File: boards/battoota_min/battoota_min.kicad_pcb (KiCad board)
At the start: 2 copper layers, 110.9 x 82.1 mm, 21 parts

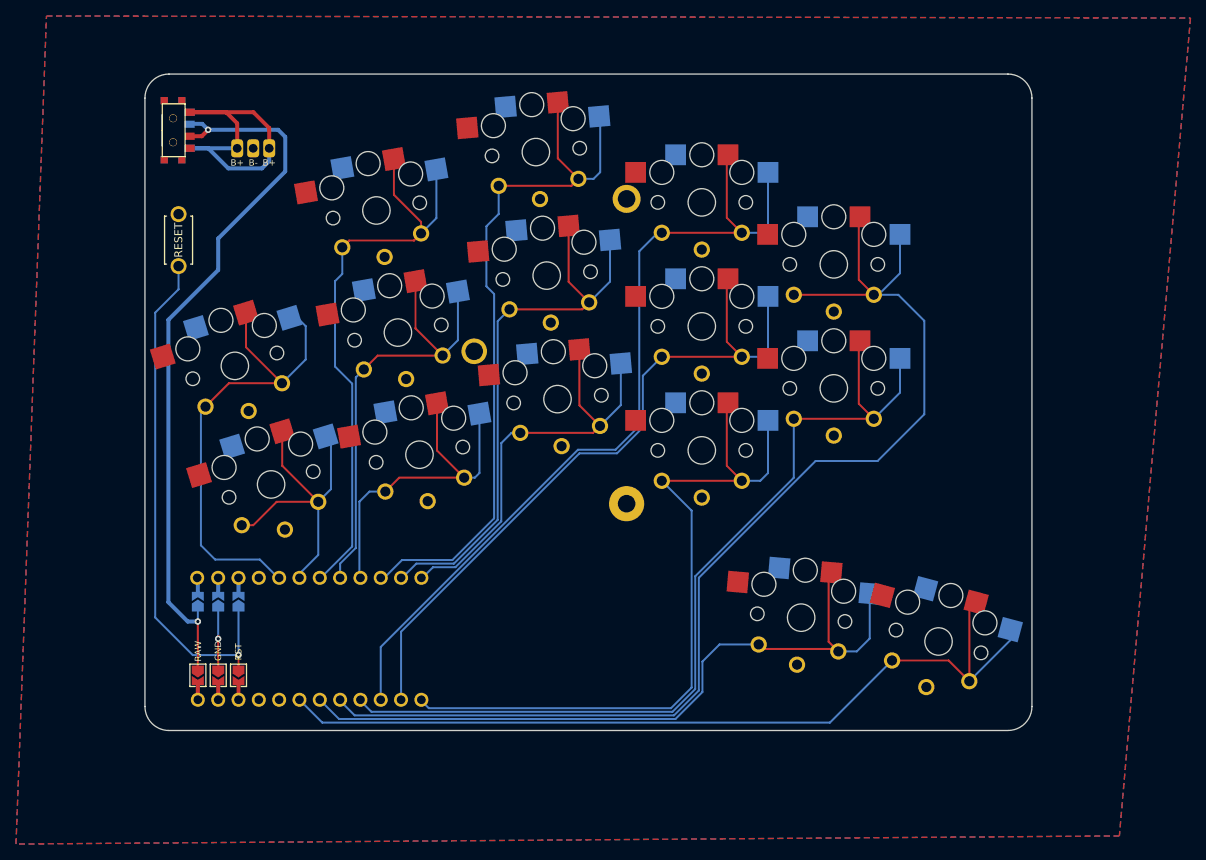
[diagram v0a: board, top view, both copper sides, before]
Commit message: min changes
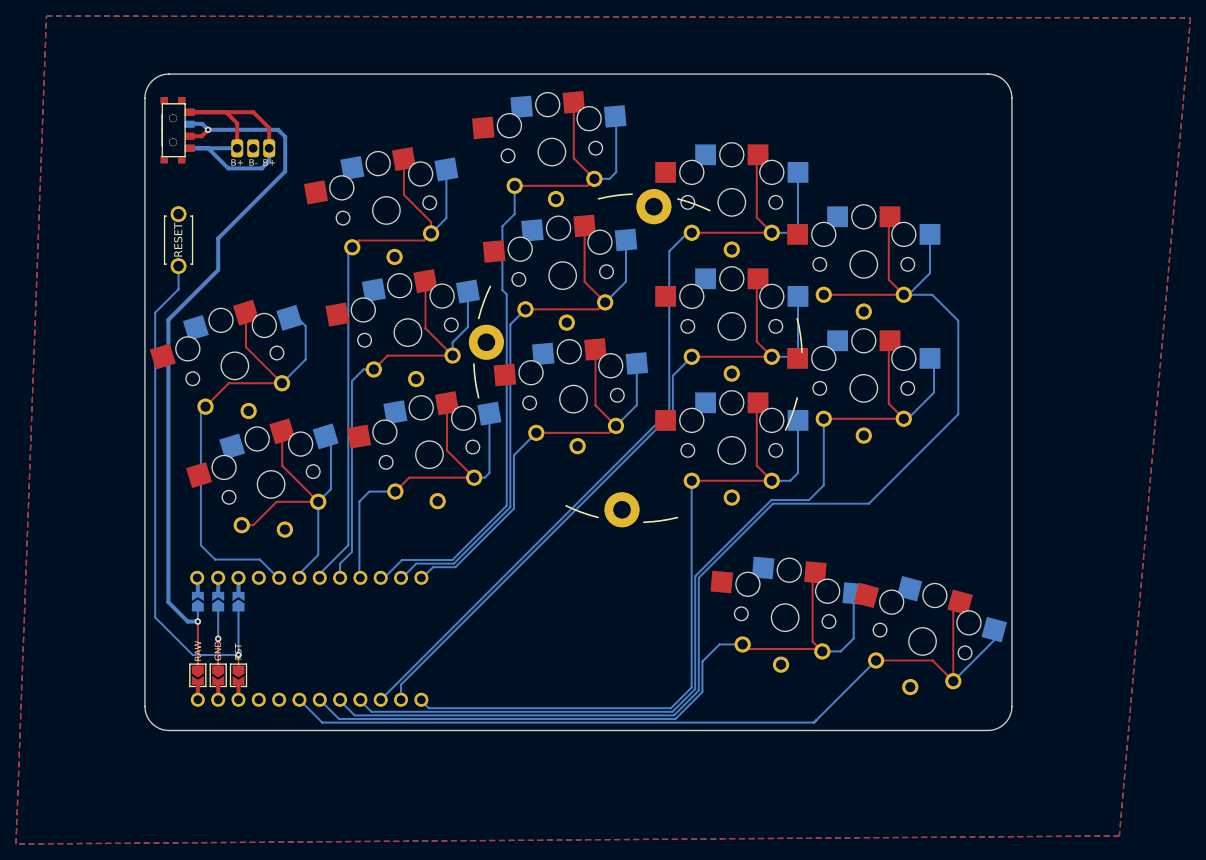
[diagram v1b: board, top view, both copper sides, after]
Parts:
- removed ?: , clipboard:26e710fa-e187-4e29-9de4-4e8ff64e7115
- added REF**: Tenting Puck, Alaa:Tenting_Puck, F.Cu at (253.1, 92.6)
- moved S10 3.75 mm to (264.9, 88.6)
- moved S11 3.75 mm to (264.9, 73.1)
- moved S12 3.75 mm to (281.4, 96.3)
- moved S13 3.75 mm to (281.4, 80.8)
- moved S9 3.75 mm to (264.9, 104.1)
- moved S14 2.00 mm to (271.5, 125.0)
- moved S15 2.00 mm to (288.7, 128.0)
- moved S6 2.00 mm to (245.1, 97.7)
- moved S7 2.00 mm to (243.7, 82.2)
- moved S8 2.00 mm to (242.4, 66.8)
- moved S3 1.25 mm to (227.1, 104.6)
- moved S4 1.25 mm to (224.4, 89.4)
- moved S5 1.25 mm to (221.7, 74.1)
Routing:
- net P5: track 146.8 -> 151.6 mm
- net P6: track 112.0 -> 116.3 mm
- net P4: track 93.0 -> 91.0 mm
- net P3: track 108.0 -> 106.4 mm
- net P9: track 93.5 -> 91.9 mm
- net P7: track 106.9 -> 105.6 mm
- net P8: track 90.2 -> 88.9 mm
- net P18: track 57.5 -> 58.7 mm
- net P19: track 74.5 -> 73.2 mm
- net P15: track 44.1 -> 45.4 mm
- net P16: track 71.9 -> 72.7 mm
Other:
- board size 110.9 x 82.1 mm -> 108.4 x 82.1 mm
